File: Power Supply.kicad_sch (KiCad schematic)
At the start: 17 parts, among them J1 Conn_01x02_Pin, J2 Conn_01x02_Pin, J3 Conn_01x03_Pin, J4 Conn_01x03_Pin, J5 Screw_Terminal_01x02, J6 Barrel_Jack, J7 Screw_Terminal_01x02, U1 LM7805_TO220, U2 LM317_TO-220

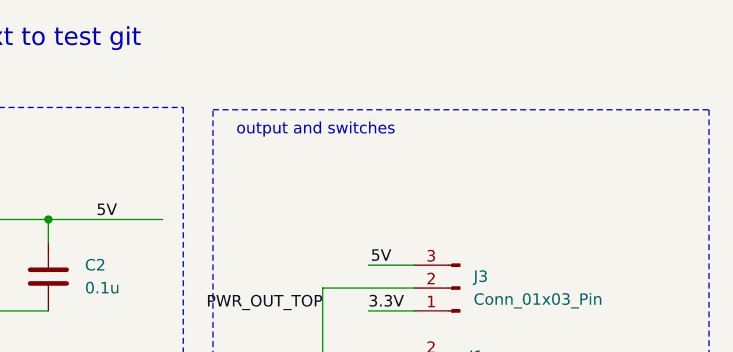
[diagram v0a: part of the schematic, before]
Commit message: added another text
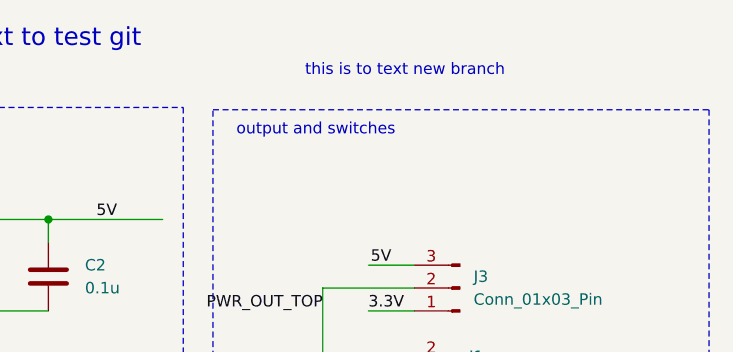
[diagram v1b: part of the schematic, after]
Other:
- note added: "this is to text new branch"
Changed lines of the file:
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@@
+		)
+	)
+	(text "this is to text new branch\n"
+		(exclude_from_sim no)
+		(at 164.084 29.21 0)
+		(effects
+			(font
+				(size 1.27 1.27)
+			)
 		)
 	)

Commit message: remove a text
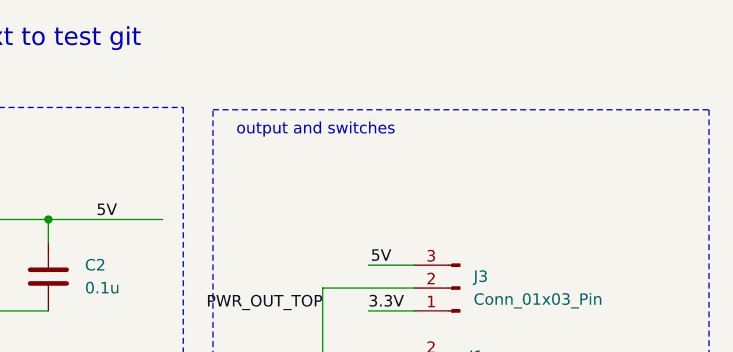
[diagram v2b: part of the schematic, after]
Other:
- note removed: "this is to text new branch"
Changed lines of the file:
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@@
-		)
-	)
-	(text "this is to text new branch\n"
-		(exclude_from_sim no)
-		(at 164.084 29.21 0)
-		(effects
-			(font
-				(size 1.27 1.27)
-			)
 		)
 	)
